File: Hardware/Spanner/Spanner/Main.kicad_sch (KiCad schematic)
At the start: 58 parts, among them J1 USB_B_Micro, J2 SWD, J3 MOTOR, J4 MOTOR, J5 MOTOR, J8 MOTOR, Q1 BC846, Q3 BC846, Q5 BC846, Q6 BC846, U1 STM32L412K8Tx, U2 USBLC6-2SC6, U3 CURRENT_SENS, U4 RFM95W-868S2, U5 MCP1812AT-033/TT, U6 OPA990

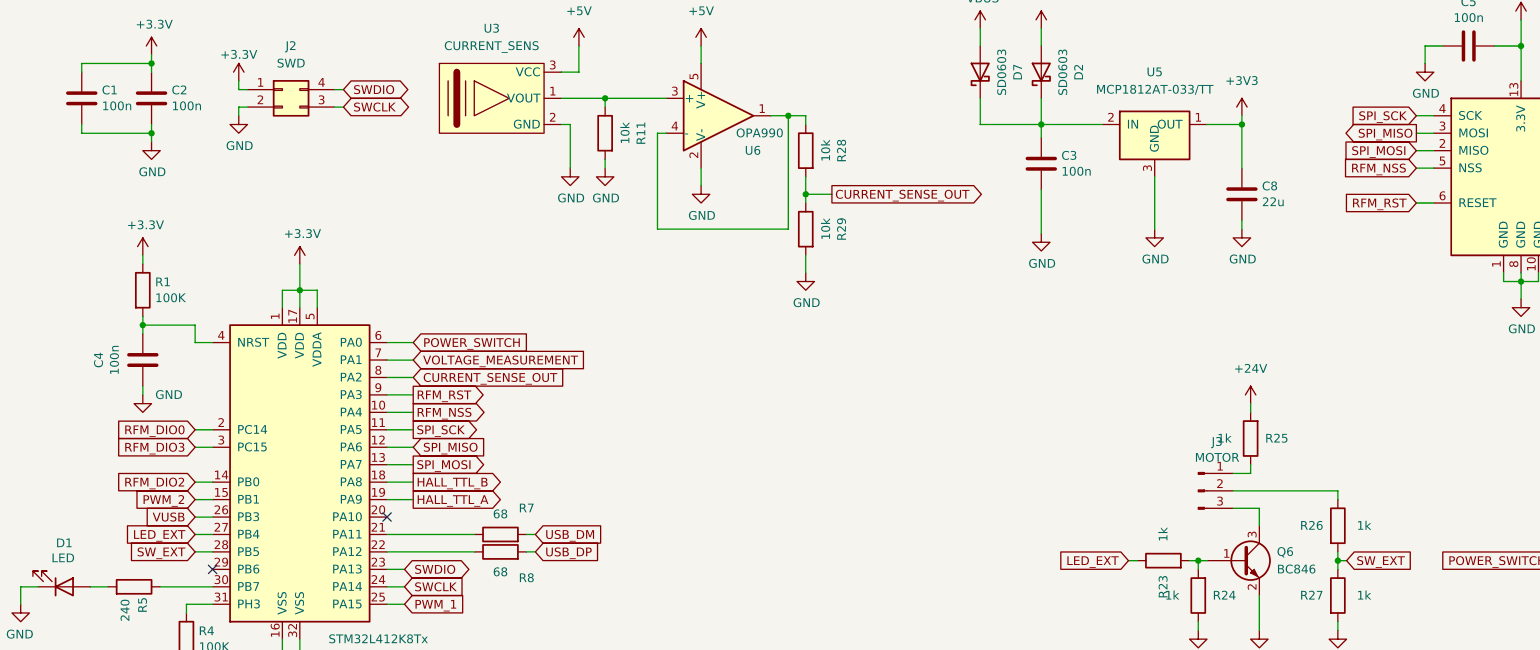
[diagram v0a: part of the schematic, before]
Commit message: update spanner
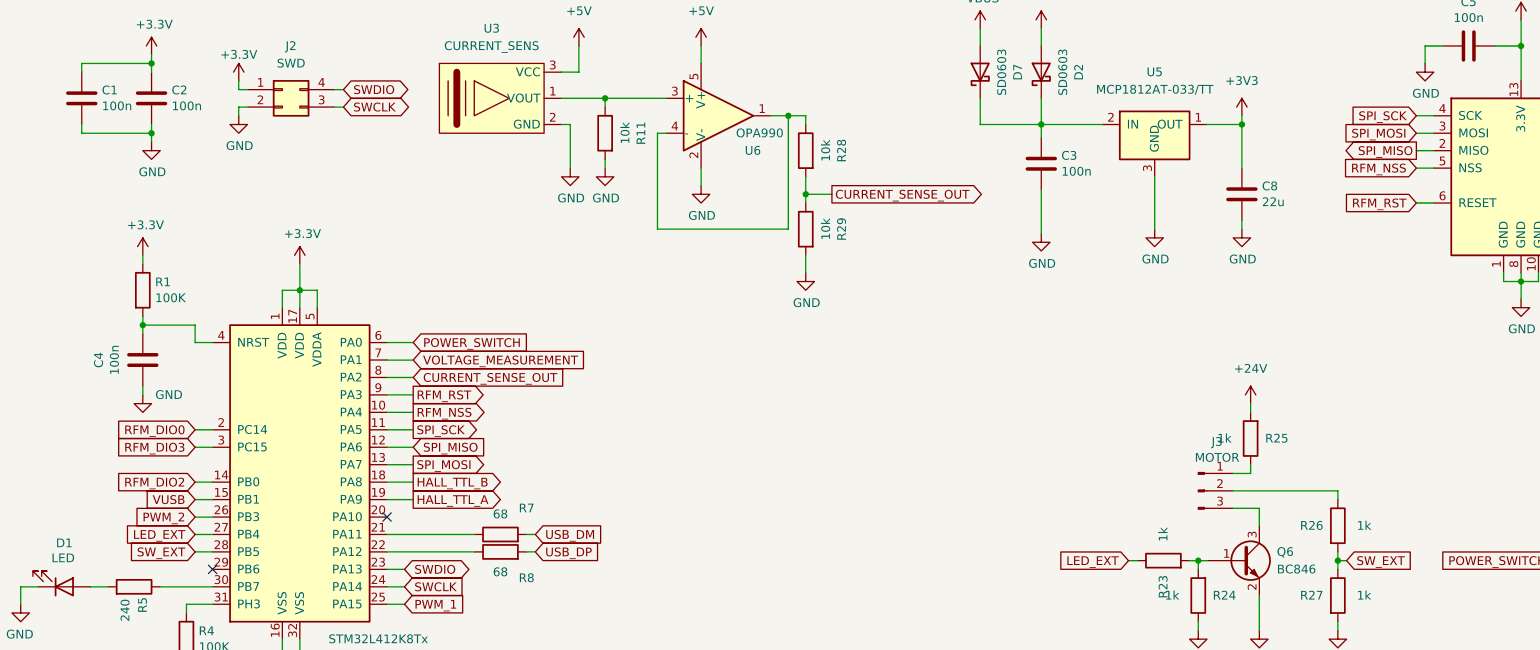
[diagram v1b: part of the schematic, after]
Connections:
- net PWM_2: now also U1.26 (PB3); no longer U1.15 (PB1)
- net SPI_MISO: now also U4.2 (MISO); no longer U4.3 (MOSI)
- net SPI_MOSI: now also U4.3 (MOSI); no longer U4.2 (MISO)
- net VUSB: now also U1.15 (PB1); no longer U1.26 (PB3)
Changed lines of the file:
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@@
     )
   )
-  (global_label "SPI_MISO" (shape output) (at 220.98 35.56 180) (fields_autoplaced)
-    (effects (font (size 1.27 1.27)) (justify right))
-    (property "Intersheet References" "${INTERSHEET_REFS}" (id 0) (at -1.27 -8.89 0)
+  (global_label "SPI_MISO" (shape output) (at 220.98 38.1 180) (fields_autoplaced)
+    (effects (font (size 1.27 1.27)) (justify right))
+    (property "Intersheet References" "${INTERSHEET_REFS}" (id 0) (at -1.27 -6.35 0)
       (effects (font (size 1.27 1.27)) hide)
     )
@@
     )
   )
-  (global_label "VUSB" (shape input) (at 43.18 91.44 180) (fields_autoplaced)
-    (effects (font (size 1.27 1.27)) (justify right))
-    (property "Intersheet References" "${INTERSHEET_REFS}" (id 0) (at 35.8683 91.5194 0)
+  (global_label "VUSB" (shape input) (at 43.18 88.9 180) (fields_autoplaced)
+    (effects (font (size 1.27 1.27)) (justify right))
+    (property "Intersheet References" "${INTERSHEET_REFS}" (id 0) (at 35.8683 88.9794 0)
       (effects (font (size 1.27 1.27)) (justify right) hide)
     )
@@
     )
   )
-  (global_label "SPI_MOSI" (shape input) (at 220.98 38.1 180) (fields_autoplaced)
-    (effects (font (size 1.27 1.27)) (justify right))
-    (property "Intersheet References" "${INTERSHEET_REFS}" (id 0) (at -1.27 -8.89 0)
+  (global_label "SPI_MOSI" (shape input) (at 220.98 35.56 180) (fields_autoplaced)
+    (effects (font (size 1.27 1.27)) (justify right))
+    (property "Intersheet References" "${INTERSHEET_REFS}" (id 0) (at -1.27 -11.43 0)
       (effects (font (size 1.27 1.27)) hide)
     )
@@
     )
   )
-  (global_label "PWM_2" (shape input) (at 43.18 88.9 180) (fields_autoplaced)
-    (effects (font (size 1.27 1.27)) (justify right))
-    (property "Intersheet References" "${INTERSHEET_REFS}" (id 0) (at 34.4169 88.8206 0)
-      (effects (font (size 1.27 1.27)) (justify right) hide)
-    )
+  (global_label "PWM_2" (shape input) (at 43.18 91.44 180) (fields_autoplaced)
+    (effects (font (size 1.27 1.27)) (justify right))
+    (property "Intersheet References" "${INTERSHEET_REFS}" (id 0) (at 34.4169 91.3606 0)
+      (effects (font (size 1.27 1.27)) (justify right) hide)
+    )
